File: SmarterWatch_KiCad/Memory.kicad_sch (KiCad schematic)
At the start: 7 parts, among them U12 M24C64-WMN6TP

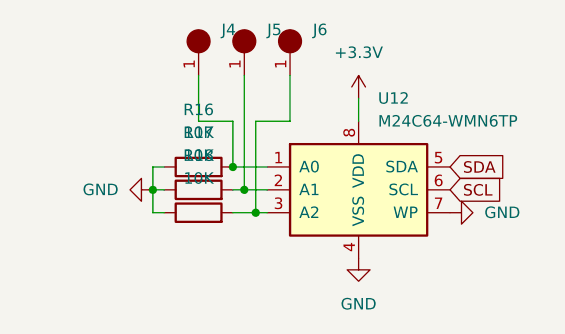
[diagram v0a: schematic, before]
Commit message: Clean Up
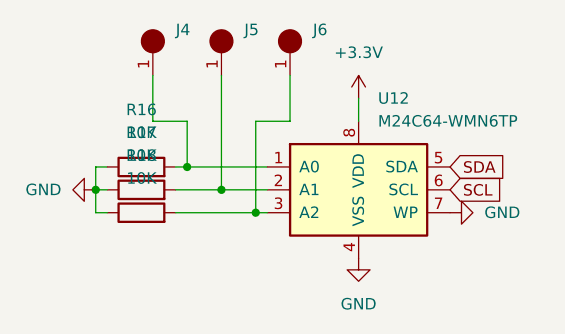
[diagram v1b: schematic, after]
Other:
- moved on the sheet: J4, J5, R16, R17, R18
